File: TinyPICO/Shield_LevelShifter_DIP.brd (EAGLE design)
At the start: 31.9 x 17.8 mm, 10 parts, among them U1 SN74HCT245N

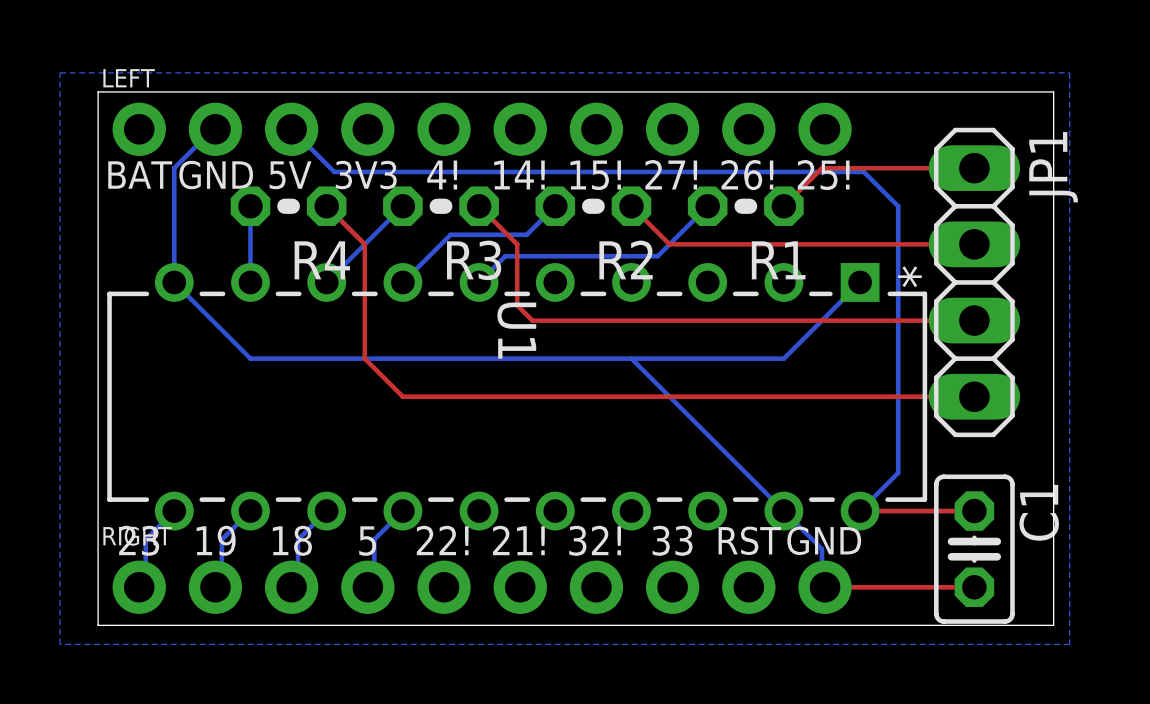
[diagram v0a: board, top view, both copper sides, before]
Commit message: Prettier
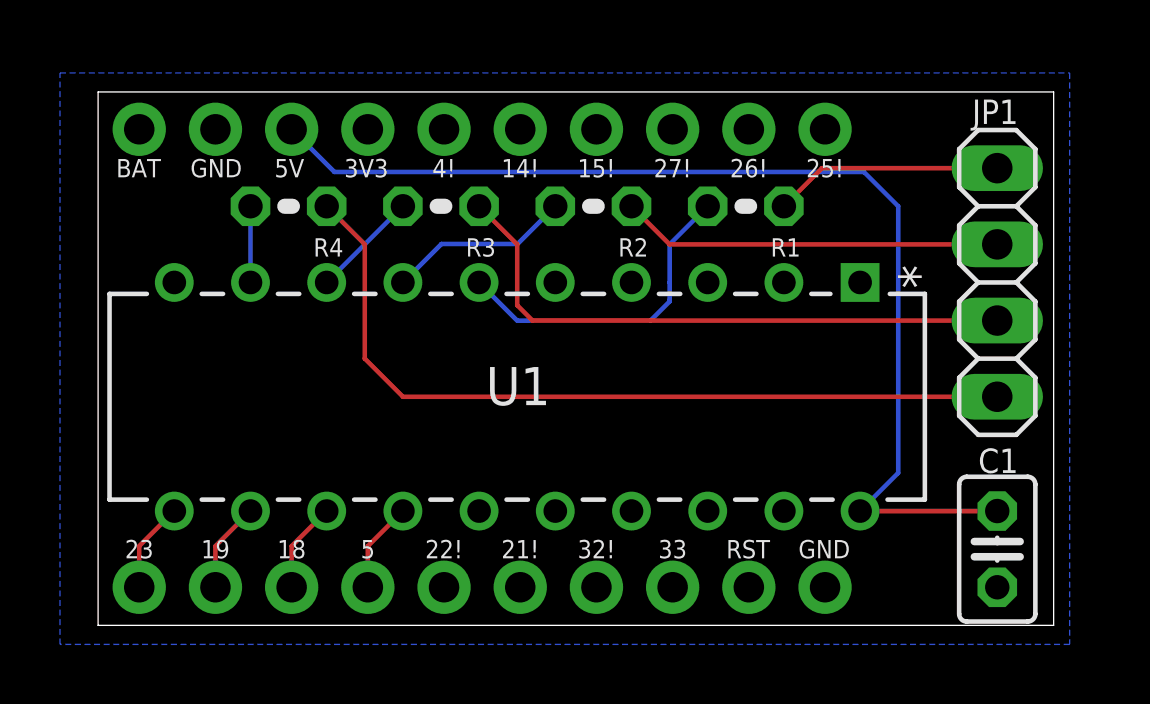
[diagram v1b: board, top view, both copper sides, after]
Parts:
- R1, R2, R3, R4: value 300 -> 300-500Ω
- moved LOGO1 22.0 mm to (7.75, 6.14), turned to 180 degrees
- moved C1 0.76 mm to (30.0, 2.54)
- moved JP1 0.76 mm to (30.0, 11.4)
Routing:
- net GND: track 46.0 -> 0.00 mm
- net N$2: track 8.67 -> 10.8 mm
- net N$13: track 26.5 -> 27.2 mm
- net N$12: track 19.3 -> 20.0 mm
- net N$11: track 12.0 -> 12.7 mm
- net N$10: track 6.88 -> 7.64 mm
- net +5V: track 36.0 -> 36.8 mm
- added copper zone on layer 16, net GND
- removed copper zone on layer 16, net GND1
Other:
- board text added: "LEVEL SHIFTER v1"
- board text removed: "LEVEL SHIFTER"
